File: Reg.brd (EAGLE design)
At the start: 30.5 x 21 mm, 28 parts, among them Q1 NPN2SC3422-2, Q2 NPN2SC3325, Q3 PNP2SA1313, Q4 NPN2SC3325, Q5 NPN2SC3422-2, Q6 NPN2SC3325, Q7 PNP2SA1313, Q8 PNP2SA1313

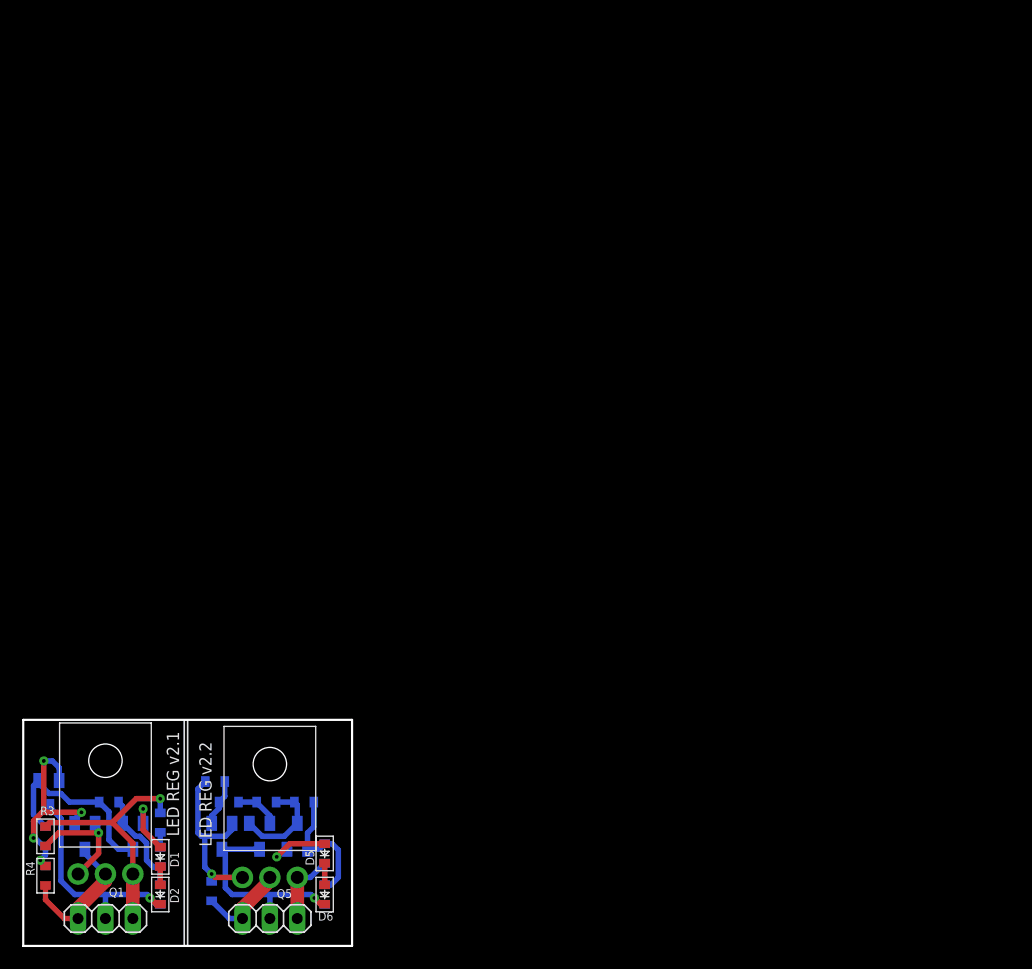
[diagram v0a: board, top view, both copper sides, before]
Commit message: Vカット
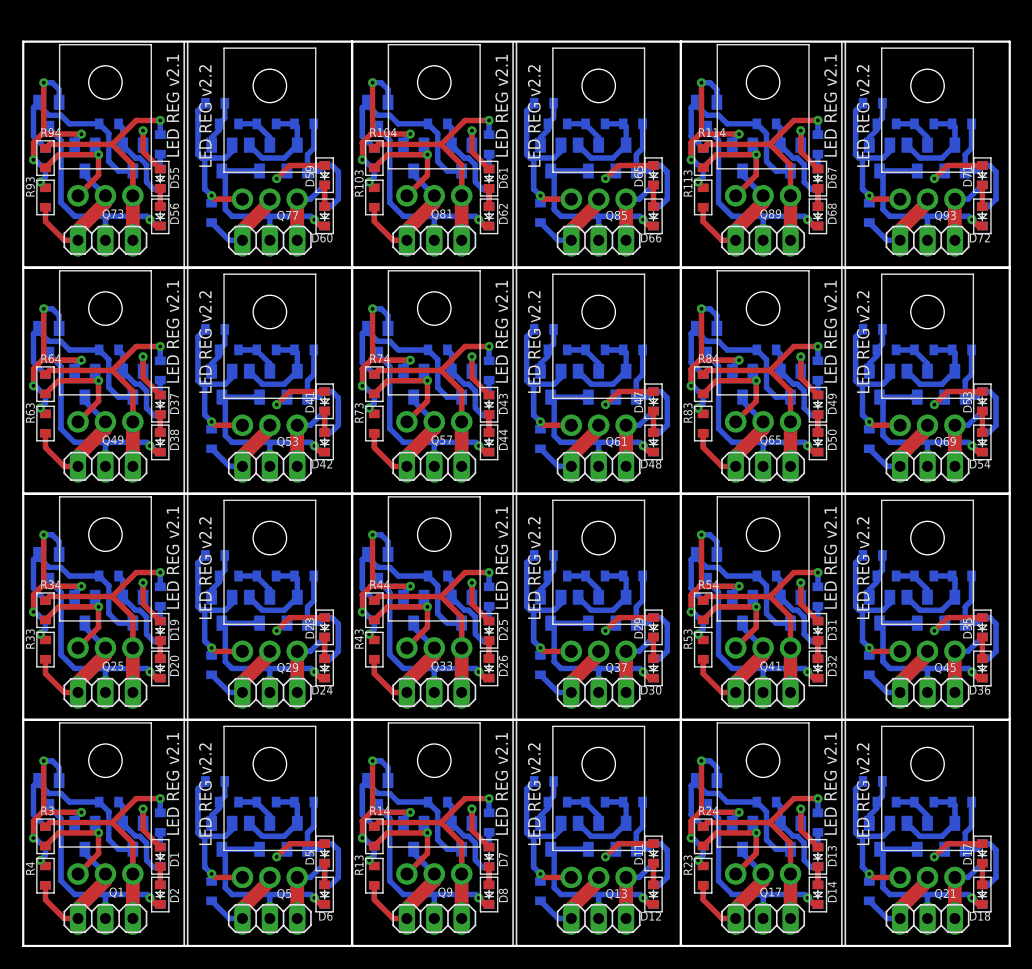
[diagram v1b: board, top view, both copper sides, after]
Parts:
- added C10, C11, C12, C13, C14, C15, C16, C17, C18, C19, C2, C20, C21, C22, C23, C24, C3, C4, C5, C6, C8, C9: 100p, my_rcl:1608
- added D10, D11, D12, D15, D16, D17, D18, D21, D22, D23, D24, D27, D28, D29, D30, D33, D34, D35, D36, D39, D40, D41, D42, D45, D46, D47, D48, D51, D52, D53, D54, D57, D58, D59, D60, D63, D64, D65, D66, D69, D70, D71, D72, D9: BLUE, my_rcl:D1608
- added D13, D14, D19, D20, D25, D26, D31, D32, D37, D38, D43, D44, D49, D50, D55, D56, D61, D62, D67, D68, D7, D8: SHORT, my_rcl:D1608
- added JP10, JP11, JP12, JP13, JP14, JP15, JP16, JP17, JP18, JP19, JP20, JP21, JP22, JP23, JP24, JP3, JP4, JP5, JP6, JP7, JP8, JP9: CON, pinhead:1X03
- added Q10, Q12, Q14, Q18, Q20, Q22, Q26, Q28, Q30, Q34, Q36, Q38, Q42, Q44, Q46, Q50, Q52, Q54, Q58, Q60, Q62, Q66, Q68, Q70, Q74, Q76, Q78, Q82, Q84, Q86, Q90, Q92, Q94: NPN2SC3325, my_ic:SC59
- added Q11, Q15, Q16, Q19, Q23, Q24, Q27, Q31, Q32, Q35, Q39, Q40, Q43, Q47, Q48, Q51, Q55, Q56, Q59, Q63, Q64, Q67, Q71, Q72, Q75, Q79, Q80, Q83, Q87, Q88, Q91, Q95, Q96: PNP2SA1313, my_ic:SC59
- added Q13, Q17, Q21, Q25, Q29, Q33, Q37, Q41, Q45, Q49, Q53, Q57, Q61, Q65, Q69, Q73, Q77, Q81, Q85, Q89, Q9, Q93: NPN2SC3422-2, my_ic:TO126-2
- added R100, R101, R102, R103, R105, R106, R107, R108, R11, R110, R111, R112, R113, R115, R116, R117, R118, R120, R13, R15, R16, R17, R18, R20, R21, R22, R23, R25, R26, R27, R28, R30, R31, R32, R33, R35, R36, R37, R38, R40, R41, R42, R43, R45, R46, R47, R48, R50, R51, R52, R53, R55, R56, R57, R58, R60, R61, R62, R63, R65, R66, R67, R68, R70, R71, R72, R73, R75, R76, R77, R78, R8, R80, R81, R82, R83, R85, R86, R87, R88, R90, R91, R92, R93, R95, R96, R97, R98: 1.5k, my_rcl:1608
- added R104, R114, R14, R24, R34, R44, R54, R64, R74, R84, R94: 10k, my_rcl:1608
- added R109, R119, R19, R29, R39, R49, R59, R69, R79, R89, R99: 0.75k, my_rcl:1608
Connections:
- new net GND10: D32.K, JP11.2, Q43.3, R51.1
- new net GND11: D36.K, JP12.2, Q47.3, Q48.3, R55.1
- new net GND12: D38.K, JP13.2, Q51.3, R61.1
- new net GND13: D42.K, JP14.2, Q55.3, Q56.3, R65.1
- new net GND14: D44.K, JP15.2, Q59.3, R71.1
- new net GND15: D48.K, JP16.2, Q63.3, Q64.3, R75.1
- new net GND16: D50.K, JP17.2, Q67.3, R81.1
- new net GND17: D54.K, JP18.2, Q71.3, Q72.3, R85.1
- new net GND18: D56.K, JP19.2, Q75.3, R91.1
- new net GND19: D60.K, JP20.2, Q79.3, Q80.3, R95.1
- new net GND2: D8.K, JP3.2, Q11.3, R8.1
- new net GND20: D62.K, JP21.2, Q83.3, R101.1
- new net GND21: D66.K, JP22.2, Q87.3, Q88.3, R105.1
- new net GND22: D68.K, JP23.2, Q91.3, R111.1
- new net GND23: D72.K, JP24.2, Q95.3, Q96.3, R115.1
- new net GND3: D12.K, JP4.2, Q15.3, Q16.3, R15.1
- new net GND4: D14.K, JP5.2, Q19.3, R21.1
- new net GND5: D18.K, JP6.2, Q23.3, Q24.3, R25.1
- new net GND6: D20.K, JP7.2, Q27.3, R31.1
- new net GND7: D24.K, JP8.2, Q31.3, Q32.3, R35.1
- new net GND8: D26.K, JP9.2, Q35.3, R41.1
- new net GND9: D30.K, JP10.2, Q39.3, Q40.3, R45.1
- new net IN10: JP11.1, Q41.2, Q44.3, R53.2
- new net IN11: JP12.1, Q45.2, R58.2
- new net IN12: JP13.1, Q49.2, Q52.3, R63.2
- new net IN13: JP14.1, Q53.2, R68.2
- new net IN14: JP15.1, Q57.2, Q60.3, R73.2
- new net IN15: JP16.1, Q61.2, R78.2
- new net IN16: JP17.1, Q65.2, Q68.3, R83.2
- new net IN17: JP18.1, Q69.2, R88.2
- new net IN18: JP19.1, Q73.2, Q76.3, R93.2
- new net IN19: JP20.1, Q77.2, R98.2
- new net IN2: JP3.1, Q12.3, Q9.2, R13.2
- new net IN20: JP21.1, Q81.2, Q84.3, R103.2
- new net IN21: JP22.1, Q85.2, R108.2
- new net IN22: JP23.1, Q89.2, Q92.3, R113.2
- new net IN23: JP24.1, Q93.2, R118.2
- new net IN3: JP4.1, Q13.2, R18.2
- new net IN4: JP5.1, Q17.2, Q20.3, R23.2
- new net IN5: JP6.1, Q21.2, R28.2
- new net IN6: JP7.1, Q25.2, Q28.3, R33.2
- new net IN7: JP8.1, Q29.2, R38.2
- new net IN8: JP9.1, Q33.2, Q36.3, R43.2
- new net IN9: JP10.1, Q37.2, R48.2
- new net N$100: D43.K, D44.A
- new net N$101: D43.A, Q58.2
- new net N$102: Q59.2, Q60.1, R72.2, R73.1
- new net N$103: C15.1, Q58.3, Q59.1, R72.1
- new net N$104: D45.A, D46.K
- new net N$105: Q57.3, Q60.2, R74.2
- new net N$106: D47.K, D48.A
- new net N$107: D47.A, Q62.2
- new net N$108: Q63.2, R76.2, R77.1
- new net N$109: C16.1, Q62.3, Q63.1, R76.1
- new net N$110: Q64.1, R77.2, R79.1
- new net N$111: Q61.3, Q64.2, R78.1, R79.2
- new net N$112: C16.2, Q62.1, R75.2, R80.1
- new net N$113: C17.2, D51.K, Q66.1, R81.2
- new net N$114: D49.K, D50.A
- new net N$115: D49.A, Q66.2
- new net N$116: Q67.2, Q68.1, R82.2, R83.1
- new net N$117: C17.1, Q66.3, Q67.1, R82.1
- new net N$118: D51.A, D52.K
- new net N$119: Q65.3, Q68.2, R84.2
- new net N$120: D53.K, D54.A
- new net N$121: D53.A, Q70.2
- new net N$122: Q71.2, R86.2, R87.1
- new net N$123: C18.1, Q70.3, Q71.1, R86.1
- new net N$124: Q72.1, R87.2, R89.1
- new net N$125: Q69.3, Q72.2, R88.1, R89.2
- new net N$126: C18.2, Q70.1, R85.2, R90.1
- new net N$127: C19.2, D57.K, Q74.1, R91.2
- new net N$128: D55.K, D56.A
- new net N$129: D55.A, Q74.2
- new net N$130: Q75.2, Q76.1, R92.2, R93.1
- new net N$131: C19.1, Q74.3, Q75.1, R92.1
- new net N$132: D57.A, D58.K
- new net N$133: Q73.3, Q76.2, R94.2
- new net N$134: D59.K, D60.A
- new net N$135: D59.A, Q78.2
- new net N$136: Q79.2, R96.2, R97.1
- new net N$137: C20.1, Q78.3, Q79.1, R96.1
- new net N$138: Q80.1, R97.2, R99.1
- new net N$139: Q77.3, Q80.2, R98.1, R99.2
- new net N$14: D7.K, D8.A
- new net N$140: C20.2, Q78.1, R100.1, R95.2
- new net N$141: C21.2, D63.K, Q82.1, R101.2
- new net N$142: D61.K, D62.A
- new net N$143: D61.A, Q82.2
- new net N$144: Q83.2, Q84.1, R102.2, R103.1
- new net N$145: C21.1, Q82.3, Q83.1, R102.1
- new net N$146: D63.A, D64.K
- new net N$147: Q81.3, Q84.2, R104.2
- new net N$148: D65.K, D66.A
- new net N$149: D65.A, Q86.2
- new net N$150: Q87.2, R106.2, R107.1
- new net N$151: C22.1, Q86.3, Q87.1, R106.1
- new net N$152: Q88.1, R107.2, R109.1
- new net N$153: Q85.3, Q88.2, R108.1, R109.2
- new net N$154: C22.2, Q86.1, R105.2, R110.1
- new net N$155: C23.2, D69.K, Q90.1, R111.2
- new net N$156: D67.K, D68.A
- new net N$157: D67.A, Q90.2
- new net N$158: Q91.2, Q92.1, R112.2, R113.1
- new net N$159: C23.1, Q90.3, Q91.1, R112.1
- new net N$160: D69.A, D70.K
- new net N$161: Q89.3, Q92.2, R114.2
- new net N$162: D71.K, D72.A
- new net N$163: D71.A, Q94.2
- new net N$164: Q95.2, R116.2, R117.1
- new net N$165: C24.1, Q94.3, Q95.1, R116.1
- new net N$166: Q96.1, R117.2, R119.1
- new net N$167: Q93.3, Q96.2, R118.1, R119.2
- new net N$168: C24.2, Q94.1, R115.2, R120.1
- new net N$17: D7.A, Q10.2
- new net N$18: Q11.2, Q12.1, R11.2, R13.1
- new net N$19: C2.1, Q10.3, Q11.1, R11.1
- new net N$20: D10.K, D9.A
- new net N$21: Q12.2, Q9.3, R14.2
- new net N$22: D11.K, D12.A
- new net N$23: D11.A, Q14.2
- new net N$24: Q15.2, R16.2, R17.1
- new net N$25: C3.1, Q14.3, Q15.1, R16.1
- new net N$26: Q16.1, R17.2, R19.1
- new net N$27: Q13.3, Q16.2, R18.1, R19.2
- new net N$28: C3.2, Q14.1, R15.2, R20.1
- new net N$29: C4.2, D15.K, Q18.1, R21.2
- new net N$30: D13.K, D14.A
- new net N$31: D13.A, Q18.2
- new net N$32: Q19.2, Q20.1, R22.2, R23.1
- new net N$33: C4.1, Q18.3, Q19.1, R22.1
- new net N$34: D15.A, D16.K
- new net N$35: Q17.3, Q20.2, R24.2
- new net N$36: D17.K, D18.A
- new net N$37: D17.A, Q22.2
- new net N$38: Q23.2, R26.2, R27.1
- new net N$39: C5.1, Q22.3, Q23.1, R26.1
- new net N$40: Q24.1, R27.2, R29.1
- new net N$41: Q21.3, Q24.2, R28.1, R29.2
- new net N$42: C5.2, Q22.1, R25.2, R30.1
- new net N$43: C6.2, D21.K, Q26.1, R31.2
- new net N$44: D19.K, D20.A
- new net N$45: D19.A, Q26.2
- new net N$46: Q27.2, Q28.1, R32.2, R33.1
- new net N$47: C6.1, Q26.3, Q27.1, R32.1
- new net N$48: D21.A, D22.K
- new net N$49: Q25.3, Q28.2, R34.2
- new net N$50: D23.K, D24.A
- new net N$51: D23.A, Q30.2
- new net N$52: Q31.2, R36.2, R37.1
- new net N$53: C8.1, Q30.3, Q31.1, R36.1
- new net N$54: Q32.1, R37.2, R39.1
- new net N$55: Q29.3, Q32.2, R38.1, R39.2
- new net N$56: C8.2, Q30.1, R35.2, R40.1
- new net N$57: C9.2, D27.K, Q34.1, R41.2
- new net N$58: D25.K, D26.A
- new net N$59: D25.A, Q34.2
- new net N$60: Q35.2, Q36.1, R42.2, R43.1
- new net N$61: C9.1, Q34.3, Q35.1, R42.1
- new net N$62: D27.A, D28.K
- new net N$63: Q33.3, Q36.2, R44.2
- new net N$64: D29.K, D30.A
- new net N$65: D29.A, Q38.2
- new net N$66: Q39.2, R46.2, R47.1
- new net N$67: C10.1, Q38.3, Q39.1, R46.1
- new net N$68: Q40.1, R47.2, R49.1
- new net N$69: Q37.3, Q40.2, R48.1, R49.2
- new net N$7: C2.2, D9.K, Q10.1, R8.2
- new net N$70: C10.2, Q38.1, R45.2, R50.1
- new net N$71: C11.2, D33.K, Q42.1, R51.2
- new net N$72: D31.K, D32.A
- new net N$73: D31.A, Q42.2
- new net N$74: Q43.2, Q44.1, R52.2, R53.1
- new net N$75: C11.1, Q42.3, Q43.1, R52.1
- new net N$76: D33.A, D34.K
- new net N$77: Q41.3, Q44.2, R54.2
- new net N$78: D35.K, D36.A
- new net N$79: D35.A, Q46.2
- new net N$80: Q47.2, R56.2, R57.1
- new net N$81: C12.1, Q46.3, Q47.1, R56.1
- new net N$82: Q48.1, R57.2, R59.1
- new net N$83: Q45.3, Q48.2, R58.1, R59.2
- new net N$84: C12.2, Q46.1, R55.2, R60.1
- new net N$85: C13.2, D39.K, Q50.1, R61.2
- new net N$86: D37.K, D38.A
- new net N$87: D37.A, Q50.2
- new net N$88: Q51.2, Q52.1, R62.2, R63.1
- new net N$89: C13.1, Q50.3, Q51.1, R62.1
- new net N$90: D39.A, D40.K
- new net N$91: Q49.3, Q52.2, R64.2
- new net N$92: D41.K, D42.A
- new net N$93: D41.A, Q54.2
- new net N$94: Q55.2, R66.2, R67.1
- new net N$95: C14.1, Q54.3, Q55.1, R66.1
- new net N$96: Q56.1, R67.2, R69.1
- new net N$97: Q53.3, Q56.2, R68.1, R69.2
- new net N$98: C14.2, Q54.1, R65.2, R70.1
- new net N$99: C15.2, D45.K, Q58.1, R71.2
- new net OUT10: D34.A, JP11.3, Q41.1, R54.1
- new net OUT11: JP12.3, Q45.1, R60.2
- new net OUT12: D40.A, JP13.3, Q49.1, R64.1
- new net OUT13: JP14.3, Q53.1, R70.2
- new net OUT14: D46.A, JP15.3, Q57.1, R74.1
- new net OUT15: JP16.3, Q61.1, R80.2
- new net OUT16: D52.A, JP17.3, Q65.1, R84.1
- new net OUT17: JP18.3, Q69.1, R90.2
- new net OUT18: D58.A, JP19.3, Q73.1, R94.1
- new net OUT19: JP20.3, Q77.1, R100.2
- new net OUT2: D10.A, JP3.3, Q9.1, R14.1
- new net OUT20: D64.A, JP21.3, Q81.1, R104.1
- new net OUT21: JP22.3, Q85.1, R110.2
- new net OUT22: D70.A, JP23.3, Q89.1, R114.1
- new net OUT23: JP24.3, Q93.1, R120.2
- new net OUT3: JP4.3, Q13.1, R20.2
- new net OUT4: D16.A, JP5.3, Q17.1, R24.1
- new net OUT5: JP6.3, Q21.1, R30.2
- new net OUT6: D22.A, JP7.3, Q25.1, R34.1
- new net OUT7: JP8.3, Q29.1, R40.2
- new net OUT8: D28.A, JP9.3, Q33.1, R44.1
- new net OUT9: JP10.3, Q37.1, R50.2
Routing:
- net OUT22: track 0.00 -> 22.7 mm, vias 0 -> 1
- net OUT18: track 0.00 -> 22.7 mm, vias 0 -> 1
- net OUT8: track 0.00 -> 22.7 mm, vias 0 -> 1
- net OUT6: track 0.00 -> 22.7 mm, vias 0 -> 1
- net OUT4: track 0.00 -> 22.7 mm, vias 0 -> 1
- net OUT20: track 0.00 -> 22.7 mm, vias 0 -> 1
- net OUT10: track 0.00 -> 22.7 mm, vias 0 -> 1
- net OUT16: track 0.00 -> 22.7 mm, vias 0 -> 1
- net OUT12: track 0.00 -> 22.7 mm, vias 0 -> 1
- net OUT2: track 0.00 -> 22.7 mm, vias 0 -> 1
- net OUT14: track 0.00 -> 22.7 mm, vias 0 -> 1
- net GND8: track 0.00 -> 20.9 mm, vias 0 -> 1
- net GND6: track 0.00 -> 20.9 mm, vias 0 -> 1
- net GND2: track 0.00 -> 20.9 mm, vias 0 -> 1
- net GND4: track 0.00 -> 20.9 mm, vias 0 -> 1
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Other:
- board size 30.5 x 21 mm -> 91.4 x 83.8 mm
- board text added: "C1"
- board text added: "C7"
- board text added: "D1"
- board text added: "D2"
- board text added: "D3"
- board text added: "D4"
- board text added: "D5"
- board text added: "D6"
- board text added: "Q1"
- board text added: "Q2"
- board text added: "Q3"
- board text added: "Q4"
- board text added: "Q5"
- board text added: "Q6"
- board text added: "Q7"
- board text added: "Q8"
- board text added: "R1"
- board text added: "R10"
- board text added: "R12"
- board text added: "R2"
- board text added: "R3"
- board text added: "R4"
- board text added: "R5"
- board text added: "R6"
- board text added: "R7"
- board text added: "R9"
